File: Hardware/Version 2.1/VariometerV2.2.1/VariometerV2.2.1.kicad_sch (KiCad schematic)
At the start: 21 parts, among them IC1 ESP32-S3-WROOM, SW1 Switch_SW_Push, SW2 Switch_SW_Push

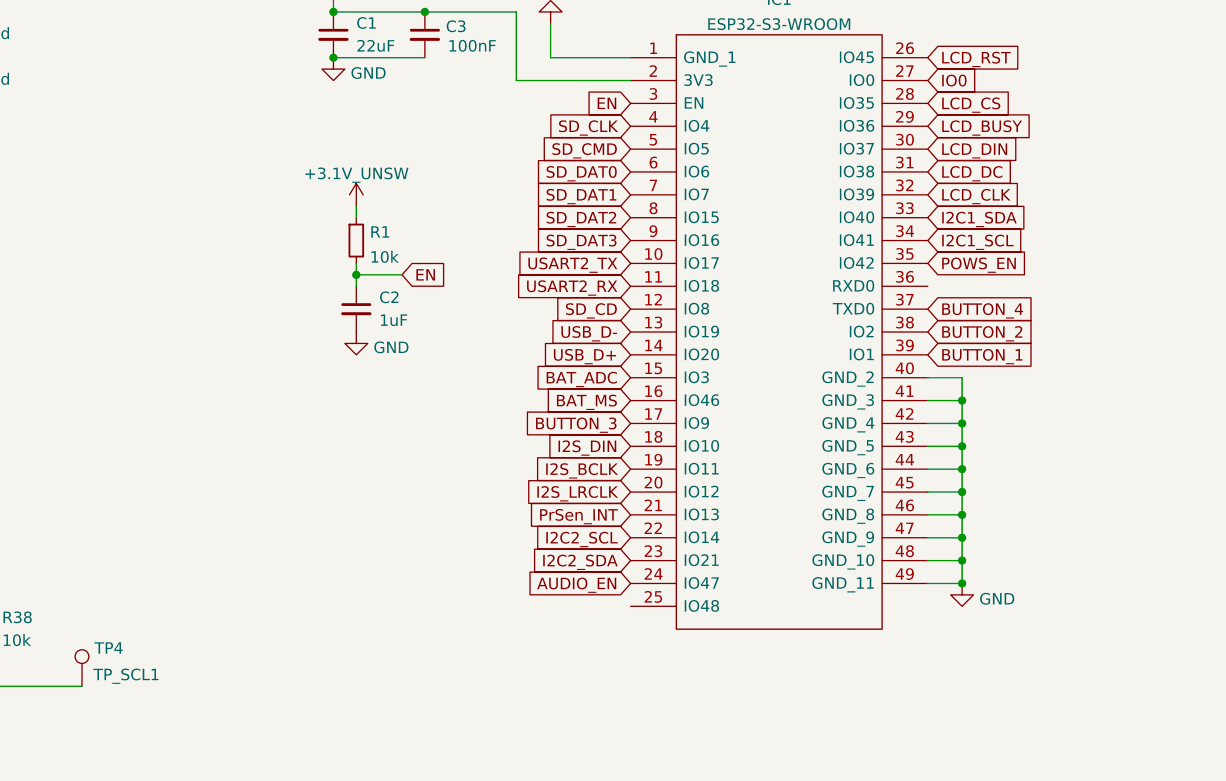
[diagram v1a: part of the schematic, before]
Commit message: Update Schematics
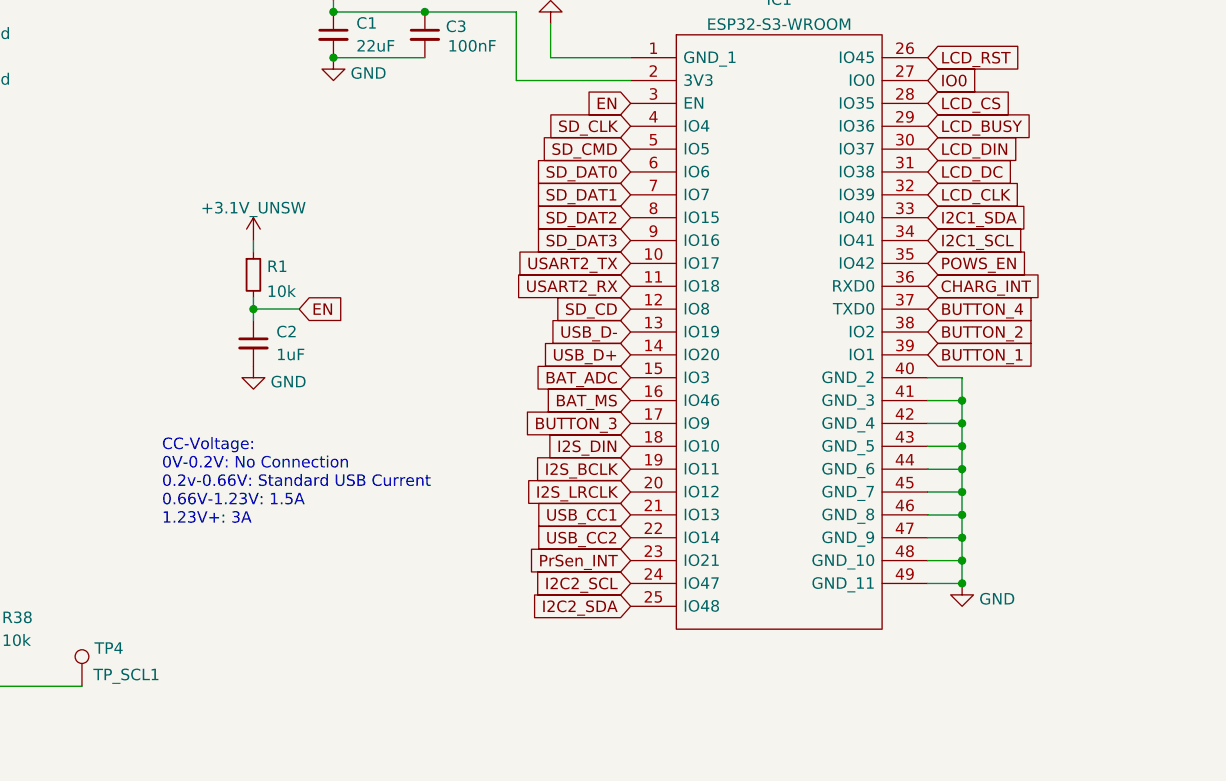
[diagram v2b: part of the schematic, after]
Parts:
- C1: footprint MainLibrary:TFP09212B -> Capacitor_SMD:C_0603_1608Metric
- C4: footprint Capacitor_SMD:C_0603_1608Metric -> Capacitor_SMD:C_0402_1005Metric
- IC1: footprint SamacSys_Parts:ESP32S3WROOM1 -> MainLibrary:ESP32S3WROOM1
- R1, R37, R38: footprint Resistor_SMD:R_0402_1005Metric -> (none)
- SW1, SW2: footprint Button_Switch_THT:SW_PUSH_6mm -> (none)
- TP3, TP4: footprint TestPoint:TestPoint_Pad_D1.5mm -> (none)
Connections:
- net AUDIO_EN is gone; now on net I2C2_SCL: IC1.24 (IO47)
- net I2C2_SCL: no longer IC1.22 (IO14)
- net I2C2_SDA: now also IC1.25 (IO48); no longer IC1.23 (IO21)
- net PrSen_INT: now also IC1.23 (IO21); no longer IC1.21 (IO13)
- net CHARG_INT: now reaches IC1.36 (RXD0)
- new net USB_CC1: IC1.21 (IO13)
- new net USB_CC2: IC1.22 (IO14)
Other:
- note added: "CC-Voltage: 0V-0.2V: No Connection 0.2v-0.66V: Standard USB Current 0.66V-1.23V: 1.5A 1.23V+: 3A"
- moved on the sheet: C2, R1

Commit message: Working on PCB
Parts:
- R1: footprint (none) -> Resistor_SMD:R_0402_1005Metric
- R37, R38: footprint (none) -> Resistor_SMD:R_0603_1608Metric
- SW1, SW2: footprint (none) -> Button_Switch_THT:SW_PUSH_6mm
- TP3, TP4: footprint (none) -> TestPoint:TestPoint_Pad_D1.5mm
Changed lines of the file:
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@@
       (effects (font (size 1.27 1.27)) (justify left))
     )
-    (property "Footprint" "" (at 66.04 167.64 0)
+    (property "Footprint" "TestPoint:TestPoint_Pad_D1.5mm" (at 66.04 167.64 0)
       (effects (font (size 1.27 1.27)) hide)
     )
@@
       (effects (font (size 1.27 1.27)) (justify left))
     )
-    (property "Footprint" "" (at 160.02 142.24 0)
+    (property "Footprint" "Button_Switch_THT:SW_PUSH_6mm" (at 160.02 142.24 0)
       (effects (font (size 1.27 1.27)) hide)
     )
@@
       (effects (font (size 1.27 1.27)) (justify left))
     )
-    (property "Footprint" "" (at 35.56 163.83 0)
+    (property "Footprint" "TestPoint:TestPoint_Pad_D1.5mm" (at 35.56 163.83 0)
       (effects (font (size 1.27 1.27)) hide)
     )
@@
       (effects (font (size 1.27 1.27)) (justify left))
     )
-    (property "Footprint" "" (at 43.18 161.29 0)
+    (property "Footprint" "Resistor_SMD:R_0603_1608Metric" (at 43.18 161.29 0)
       (effects (font (size 1.27 1.27)) hide)
     )
@@
       (effects (font (size 1.27 1.27)) (justify left))
     )
-    (property "Footprint" "" (at 50.8 161.29 0)
+    (property "Footprint" "Resistor_SMD:R_0603_1608Metric" (at 50.8 161.29 0)
       (effects (font (size 1.27 1.27)) hide)
     )
@@
       (effects (font (size 1.27 1.27)) (justify left))
     )
-    (property "Footprint" "" (at 119.38 143.51 0)
+    (property "Footprint" "Button_Switch_THT:SW_PUSH_6mm" (at 119.38 143.51 0)
       (effects (font (size 1.27 1.27)) hide)
     )
@@
       (effects (font (size 1.27 1.27)) (justify left))
     )
-    (property "Footprint" "" (at 66.04 120.65 0)
+    (property "Footprint" "TestPoint:TestPoint_Pad_D1.5mm" (at 66.04 120.65 0)
       (effects (font (size 1.27 1.27)) hide)
     )
@@
       (effects (font (size 1.27 1.27)) (justify left))
     )
-    (property "Footprint" "" (at 43.18 114.3 0)
+    (property "Footprint" "Resistor_SMD:R_0603_1608Metric" (at 43.18 114.3 0)
       (effects (font (size 1.27 1.27)) hide)
     )
@@
       (effects (font (size 1.27 1.27)) (justify left))
     )
-    (property "Footprint" "" (at 35.56 116.84 0)
+    (property "Footprint" "TestPoint:TestPoint_Pad_D1.5mm" (at 35.56 116.84 0)
       (effects (font (size 1.27 1.27)) hide)
     )
@@
       (effects (font (size 1.27 1.27)) (justify left))
     )
-    (property "Footprint" "" (at 80.01 74.93 0)
+    (property "Footprint" "Resistor_SMD:R_0402_1005Metric" (at 80.01 74.93 0)
       (effects (font (size 1.27 1.27)) hide)
     )
@@
       (effects (font (size 1.27 1.27)) (justify left))
     )
-    (property "Footprint" "" (at 50.8 114.3 0)
-      (effects (font (size 1.27 1.27)) hide)
-    )
+    (property "Footprint" "Resistor_SMD:R_0603_1608Metric" (at 50.8 114.3 0)
+      (effects (font (size 1.27 1.27)) hide)
+    )

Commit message: PCB
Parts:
- C1: JLCPCB Part # C59461 -> (none); LCSC Part (none) -> C59461
- C2: JLCPCB Part # C52923 -> (none); LCSC Part (none) -> C52923; LCSC Part # C2345 -> (none)
- C3, C5: JLCPCB Part # C307331 -> (none); LCSC Part (none) -> C307331
- C4: JLCPCB Part # C14663 -> (none); LCSC Part (none) -> C307331
- IC1: JLCPCB Part # C2913198 -> (none); LCSC Part (none) -> C2913198
- R1: JLCPCB Part # C25744 -> (none); LCSC Part (none) -> C25744
- R37, R38: JLCPCB Part # C25744 -> (none); LCSC Part (none) -> C25804
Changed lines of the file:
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@@
+      (effects (font (size 1.27 1.27)) hide)
+    )
+    (property "LCSC Part" "" (at 60.96 167.64 0)
       (effects (font (size 1.27 1.27)) hide)
     )
@@
     )
     (property "Datasheet" "" (at 160.02 142.24 0)
+      (effects (font (size 1.27 1.27)) hide)
+    )
+    (property "LCSC Part" "" (at 154.94 142.24 0)
       (effects (font (size 1.27 1.27)) hide)
     )
@@
       (effects (font (size 1.27 1.27)) hide)
     )
+    (property "LCSC Part" "" (at 30.48 163.83 0)
+      (effects (font (size 1.27 1.27)) hide)
+    )
     (pin "1")
     (instances
@@
       (effects (font (size 1.27 1.27)) hide)
     )
-    (property "JLCPCB Part #" "C25744" (at 43.18 161.29 0)
+    (property "LCSC Part" "C25804" (at 43.18 161.29 0)
       (effects (font (size 1.27 1.27)) hide)
     )
@@
       (effects (font (size 1.27 1.27)) hide)
     )
-    (property "JLCPCB Part #" "C25744" (at 50.8 161.29 0)
+    (property "LCSC Part" "C25804" (at 50.8 161.29 0)
       (effects (font (size 1.27 1.27)) hide)
     )
@@
       (effects (font (size 1.27 1.27)) (justify left) hide)
     )
-    (property "JLCPCB Part #" "C2913198" (at 121.92 50.8 0)
+    (property "LCSC Part" "C2913198" (at 121.92 50.8 0)
       (effects (font (size 1.27 1.27)) hide)
     )
@@
       (effects (font (size 1.27 1.27)) hide)
     )
+    (property "LCSC Part" "" (at 114.3 143.51 0)
+      (effects (font (size 1.27 1.27)) hide)
+    )
     (pin "1")
     (pin "2")
@@
     )
     (property "Datasheet" "~" (at 33.02 41.91 0)
+      (effects (font (size 1.27 1.27)) hide)
+    )
+    (property "LCSC Part" "" (at 33.02 41.91 0)
       (effects (font (size 1.27 1.27)) hide)
     )
@@
       (effects (font (size 1.27 1.27)) hide)
     )
+    (property "LCSC Part" "" (at 60.96 120.65 0)
+      (effects (font (size 1.27 1.27)) hide)
+    )
     (pin "1")
     (instances
@@
     )
     (property "Datasheet" "~" (at 33.02 46.99 0)
+      (effects (font (size 1.27 1.27)) hide)
+    )
+    (property "LCSC Part" "" (at 33.02 46.99 0)
       (effects (font (size 1.27 1.27)) hide)
     )
@@
       (effects (font (size 1.27 1.27)) hide)
     )
-    (property "JLCPCB Part #" "C25744" (at 43.18 114.3 0)
+    (property "LCSC Part" "C25804" (at 43.18 114.3 0)
       (effects (font (size 1.27 1.27)) hide)
     )
@@
       (effects (font (size 1.27 1.27)) hide)
     )
-    (property "JLCPCB Part #" "C14663" (at 107.95 143.51 0)
+    (property "LCSC Part" "C307331" (at 107.95 143.51 0)
       (effects (font (size 1.27 1.27)) hide)
     )
@@
       (effects (font (size 1.27 1.27)) hide)
     )
+    (property "LCSC Part" "" (at 30.48 116.84 0)
+      (effects (font (size 1.27 1.27)) hide)
+    )
     (pin "1")
     (instances
@@
       (effects (font (size 1.27 1.27)) hide)
     )
-    (property "JLCPCB Part #" "C25744" (at 80.01 74.93 0)
+    (property "LCSC Part" "C25744" (at 80.01 74.93 0)
       (effects (font (size 1.27 1.27)) hide)
     )
@@
       (effects (font (size 1.27 1.27)) hide)
     )
+    (property "LCSC Part" "" (at 33.02 36.83 0)
+      (effects (font (size 1.27 1.27)) hide)
+    )
     (pin "1")
     (instances
@@
       (effects (font (size 1.27 1.27)) hide)
     )
-    (property "JLCPCB Part #" "C307331" (at 99.06 48.26 0)
+    (property "LCSC Part" "C307331" (at 99.06 48.26 0)
       (effects (font (size 1.27 1.27)) hide)
     )
@@
       (effects (font (size 1.27 1.27)) hide)
     )
-    (property "JLCPCB Part #" "C52923" (at 80.01 82.55 0)
-      (effects (font (size 1.27 1.27)) hide)
-    )
-    (property "LCSC Part #" "C2345" (at 80.01 82.55 0)
+    (property "LCSC Part" "C52923" (at 80.01 82.55 0)
       (effects (font (size 1.27 1.27)) hide)
     )
@@
       (effects (font (size 1.27 1.27)) hide)
     )
-    (property "JLCPCB Part #" "C25744" (at 50.8 114.3 0)
+    (property "LCSC Part" "C25804" (at 50.8 114.3 0)
       (effects (font (size 1.27 1.27)) hide)
     )
@@
       (effects (font (size 1.27 1.27)) hide)
     )
-    (property "JLCPCB Part #" "C59461" (at 88.9 48.26 0)
+    (property "LCSC Part" "C59461" (at 88.9 48.26 0)
       (effects (font (size 1.27 1.27)) hide)
     )
@@
       (effects (font (size 1.27 1.27)) hide)
     )
-    (property "JLCPCB Part #" "C307331" (at 148.59 142.24 0)
+    (property "LCSC Part" "C307331" (at 148.59 142.24 0)
       (effects (font (size 1.27 1.27)) hide)
     )
@@
       (effects (font (size 1.27 1.27)) hide)
     )
+    (property "LCSC Part" "" (at 33.02 52.07 0)
+      (effects (font (size 1.27 1.27)) hide)
+    )
